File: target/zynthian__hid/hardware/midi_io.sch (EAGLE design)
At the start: 5 parts, among them IC1 74AC00N, IC2 74AC00N

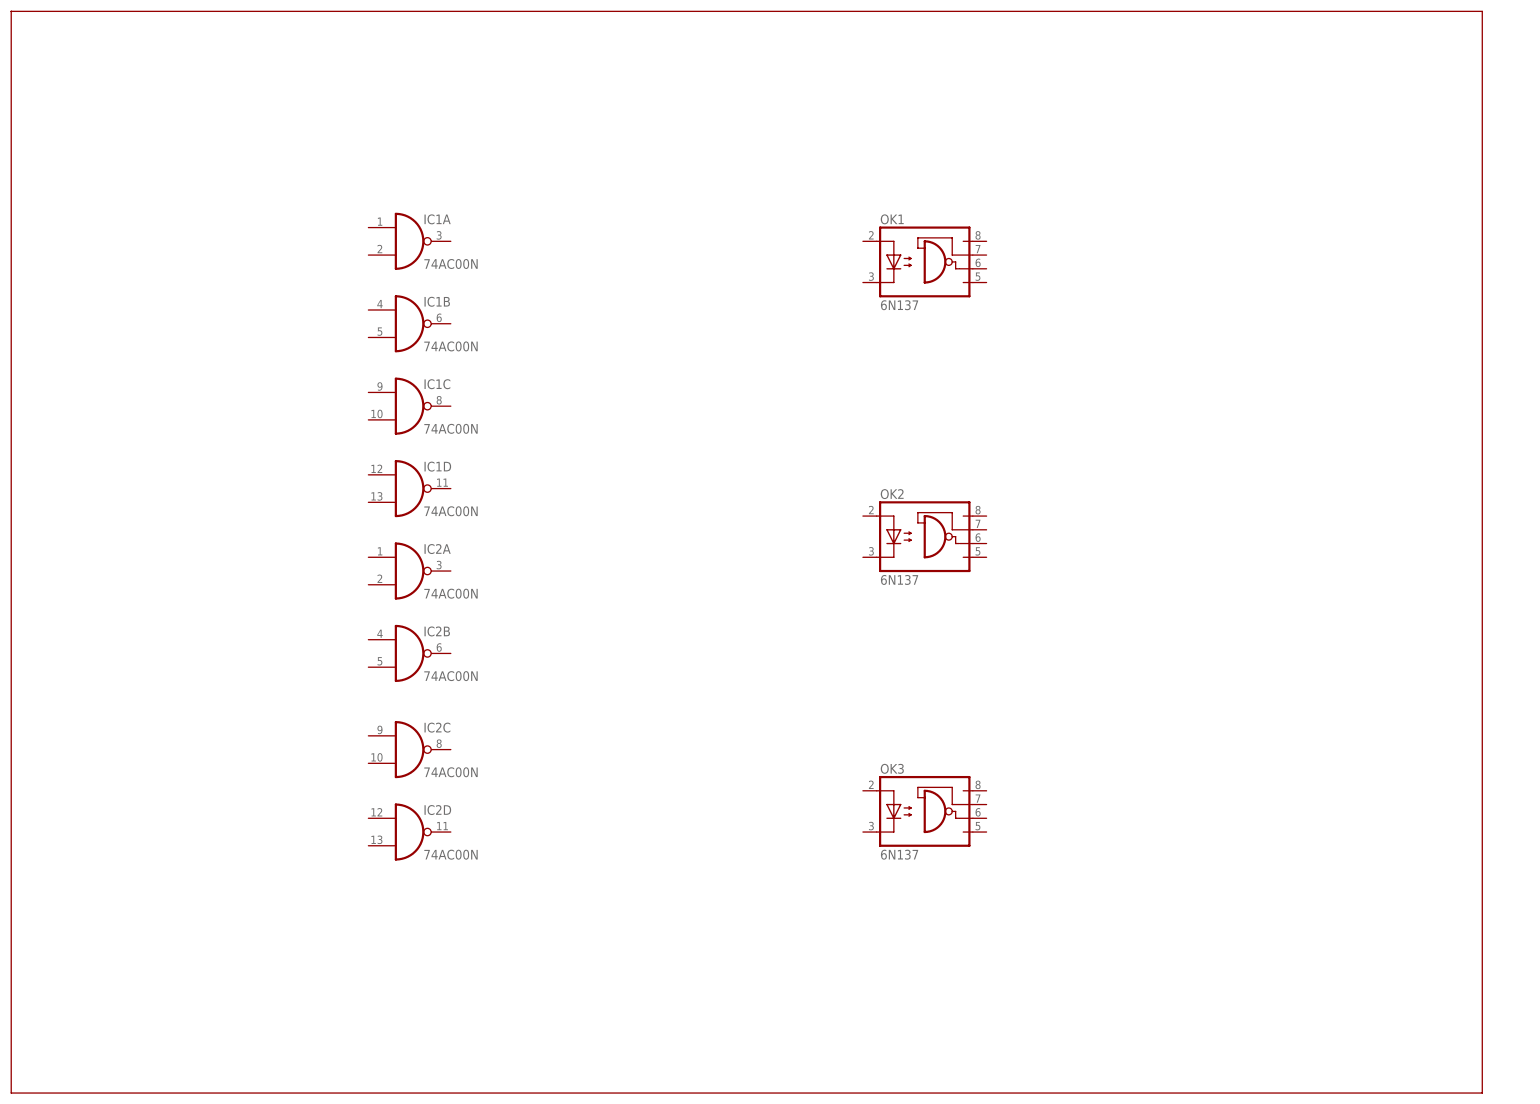
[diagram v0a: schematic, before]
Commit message: zynthian__hid: updated hardware
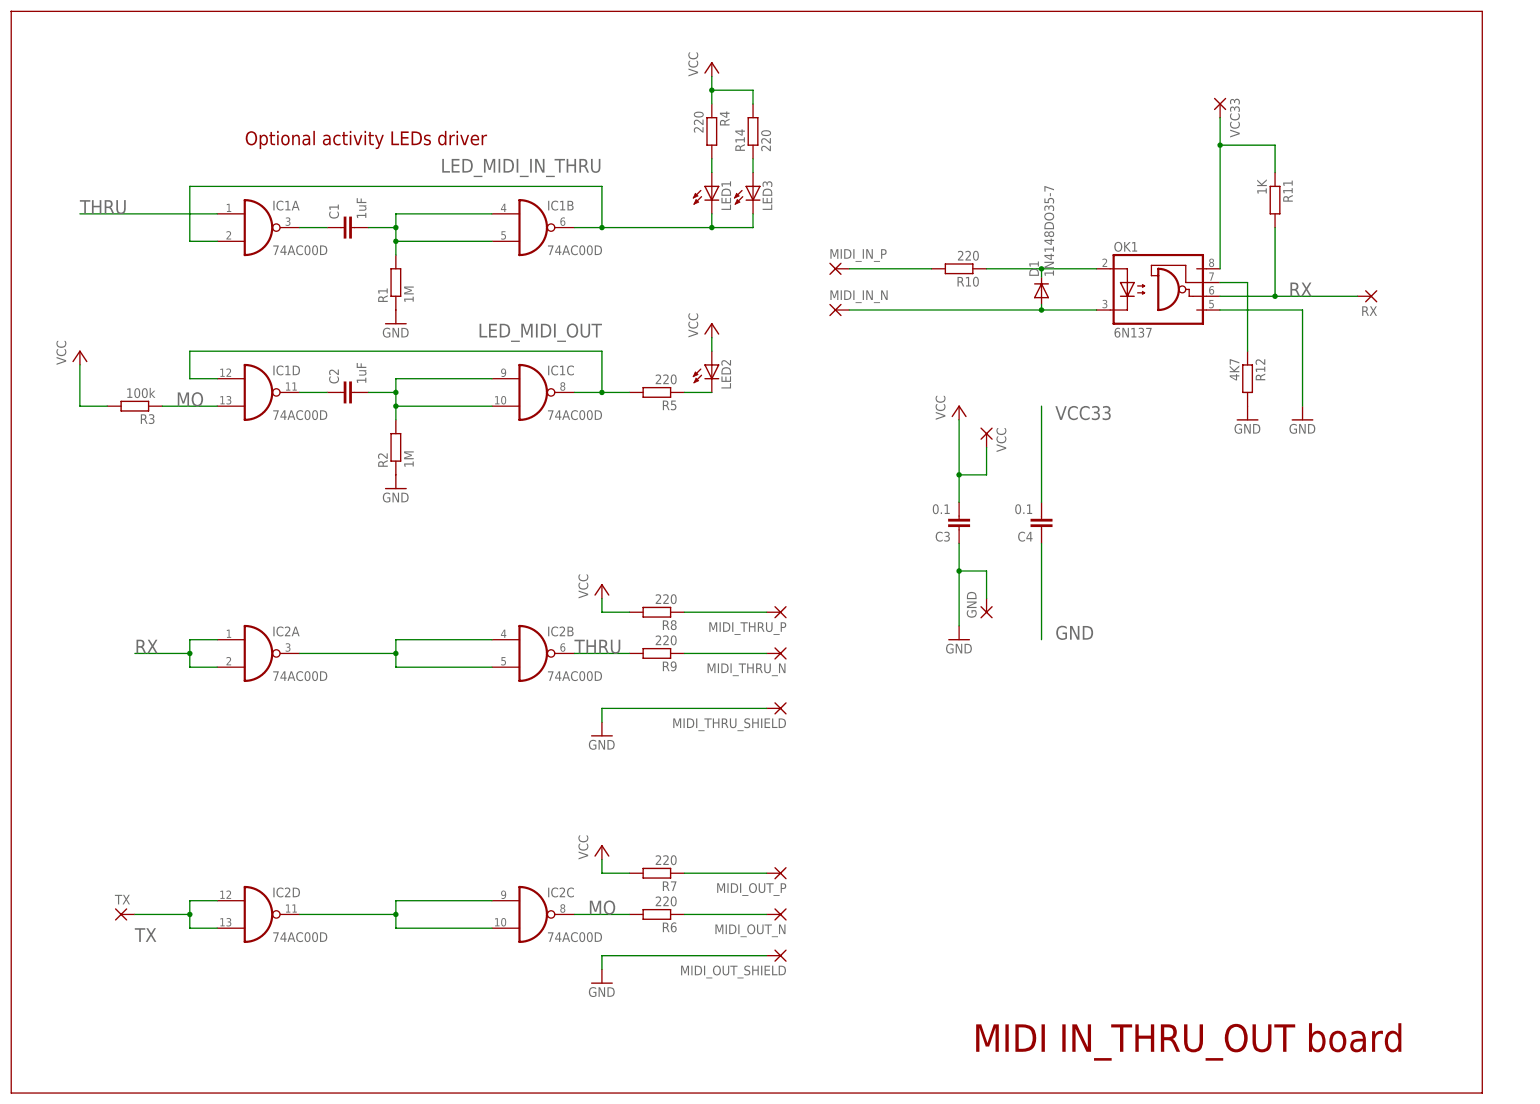
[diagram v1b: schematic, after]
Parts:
- removed OK2, OK3: 6N137, optocoupler:6N137
- added C1, C2: 1uF, rcl:C-EUC0805
- added C3, C4: 0.1, rcl:C-EUC0805
- added D1: 1N4148DO35-7, diode:1N4148DO35-7
- added GND, MIDI_IN_N, MIDI_IN_P, MIDI_OUT_N, MIDI_OUT_P, MIDI_OUT_SHIELD, MIDI_THRU_N, MIDI_THRU_P, MIDI_THRU_SHIELD, RX, TX, VCC, VCC33: (no value), wirepad:1,6/0,8
- added LED1, LED2, LED3: (no value), led:LED3MM
- added R1, R2: 1M, rcl:R-EU_M0805
- added R10, R4, R6, R7, R8, R9: 220, rcl:R-EU_0204/7
- added R11: 1K, rcl:R-EU_0204/7
- added R12: 4K7, rcl:R-EU_0204/7
- added R14: 220, rcl:R-EU_0617/17
- added R3: 100k, rcl:R-EU_M0805
- added R5: 220, rcl:R-EU_M0805
- IC1, IC2: value 74AC00N -> 74AC00D; device 74xx-eu:74AC00N -> 74xx-eu:74AC00D
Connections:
- new net GND: C3.1, C4.1, GND.P, MIDI_OUT_SHIELD.P, MIDI_THRU_SHIELD.P, OK1.GND, R1.1, R12.2, R2.1
- new net INV1: IC2A.O, IC2B.I0, IC2B.I1
- new net INV2: IC2C.I0, IC2C.I1, IC2D.O
- new net L2: LED2.C, R5.1
- new net LED_MIDI_IN_THRU: IC1A.I1, IC1B.O, LED1.C, LED3.C
- new net LED_MIDI_OUT: IC1C.O, IC1D.I0, R5.2
- new net MIDI_THRU_N: MIDI_THRU_N.P, R9.1
- new net MIDI_THRU_P: MIDI_THRU_P.P, R8.1
- new net MIDI_TX_N: MIDI_OUT_N.P, R6.1
- new net MIDI_TX_P: MIDI_OUT_P.P, R7.1
- new net MO: IC1D.I1, IC2C.O, R3.1, R6.2
- new net N$1: OK1.VE, R12.1
- new net N$2: LED1.A, R4.2
- new net N$4: LED3.A, R14.1
- new net N$5: D1.C, OK1.A, R10.1
- new net N$6: D1.A, MIDI_IN_N.P, OK1.C
- new net N$7: MIDI_IN_P.P, R10.2
- new net RC1: C1.2, IC1B.I0, IC1B.I1, R1.2
- new net RC2: C2.2, IC1C.I0, IC1C.I1, R2.2
- new net RX: IC2A.I0, IC2A.I1, OK1.VO, R11.2, RX.P
- new net THRU: IC1A.I0, IC2B.O, R9.2
- new net TO_C1: C1.1, IC1A.O
- new net TO_C2: C2.1, IC1D.O
- new net TX: IC2D.I0, IC2D.I1, TX.P
- new net VCC: C3.2, LED2.A, R14.2, R3.2, R4.1, R7.2, R8.2, VCC.P
- new net VCC33: C4.2, OK1.VCC, R11.1, VCC33.P
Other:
- note added: "MIDI IN_THRU_OUT board"
- note added: "Optional activity LEDs driver"
- moved on the sheet: IC1A, IC1B, IC1C, IC1D, IC2A, IC2B, IC2C, IC2D, OK1
